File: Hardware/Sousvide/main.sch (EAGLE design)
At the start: 14 parts, among them K1 CQ1-12V, SW1 EC12E_SW, T1 2N3904

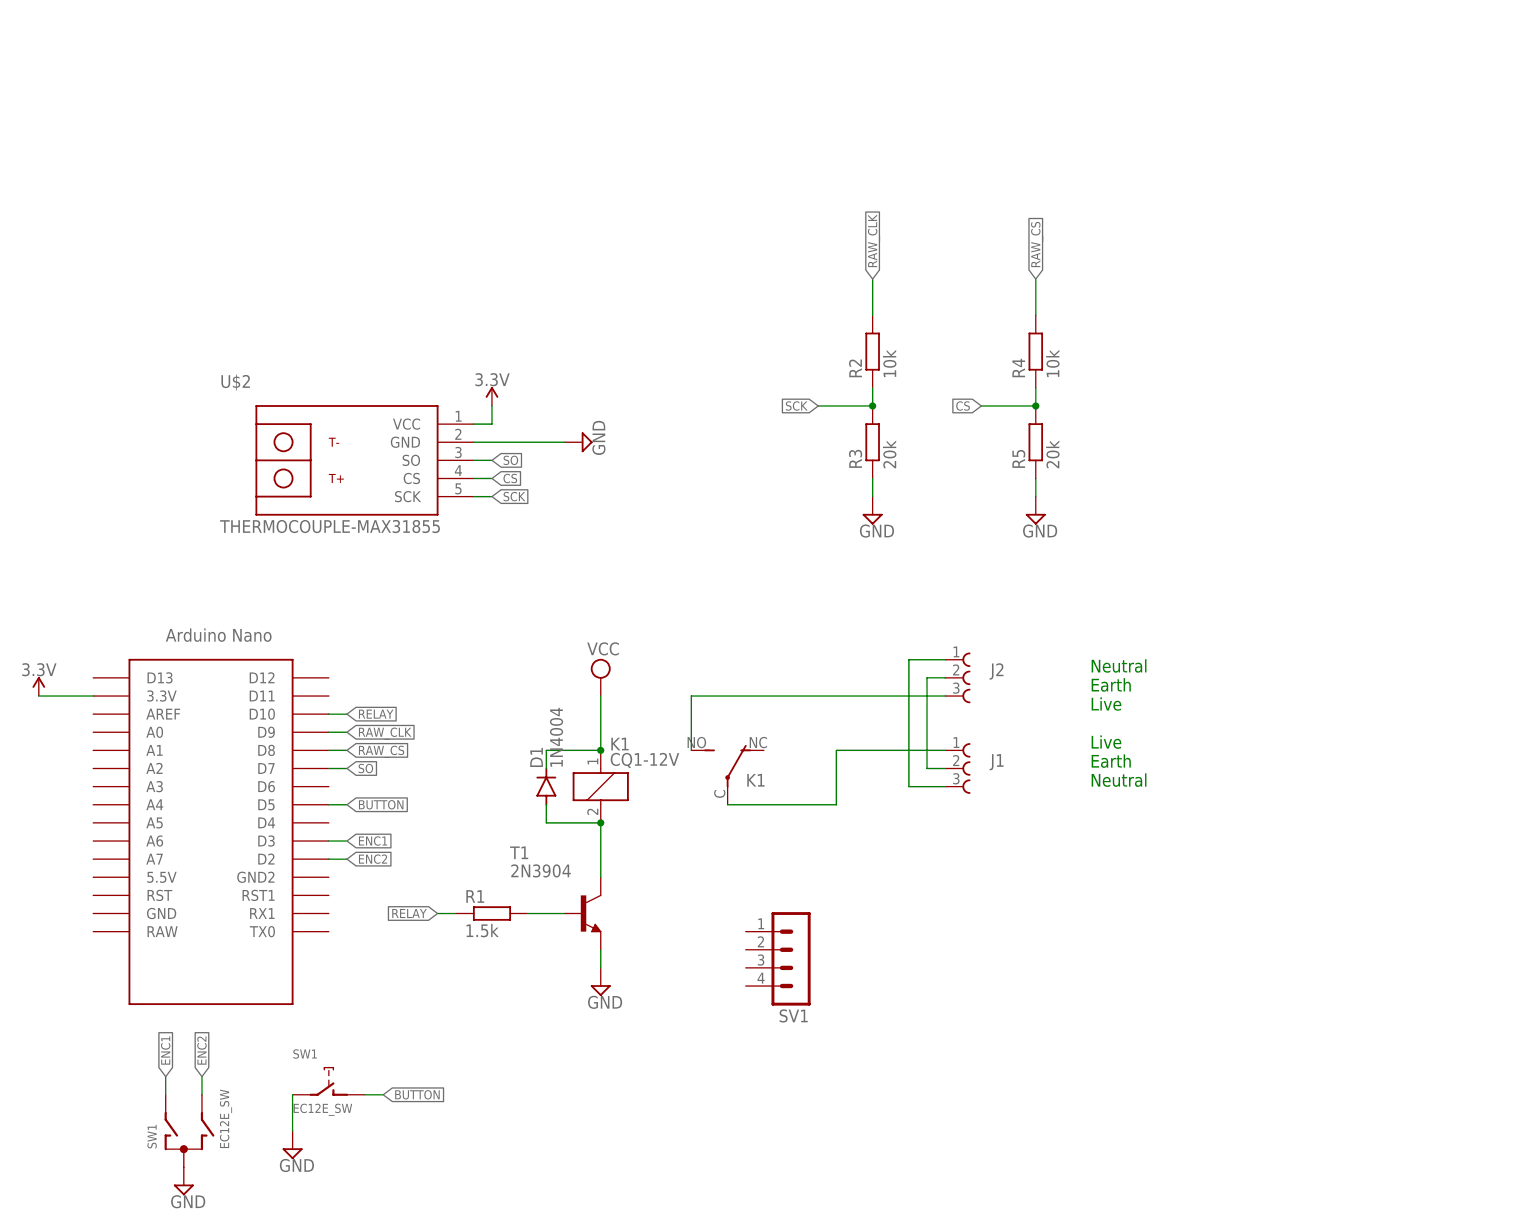
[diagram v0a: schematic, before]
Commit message: Completed schematic
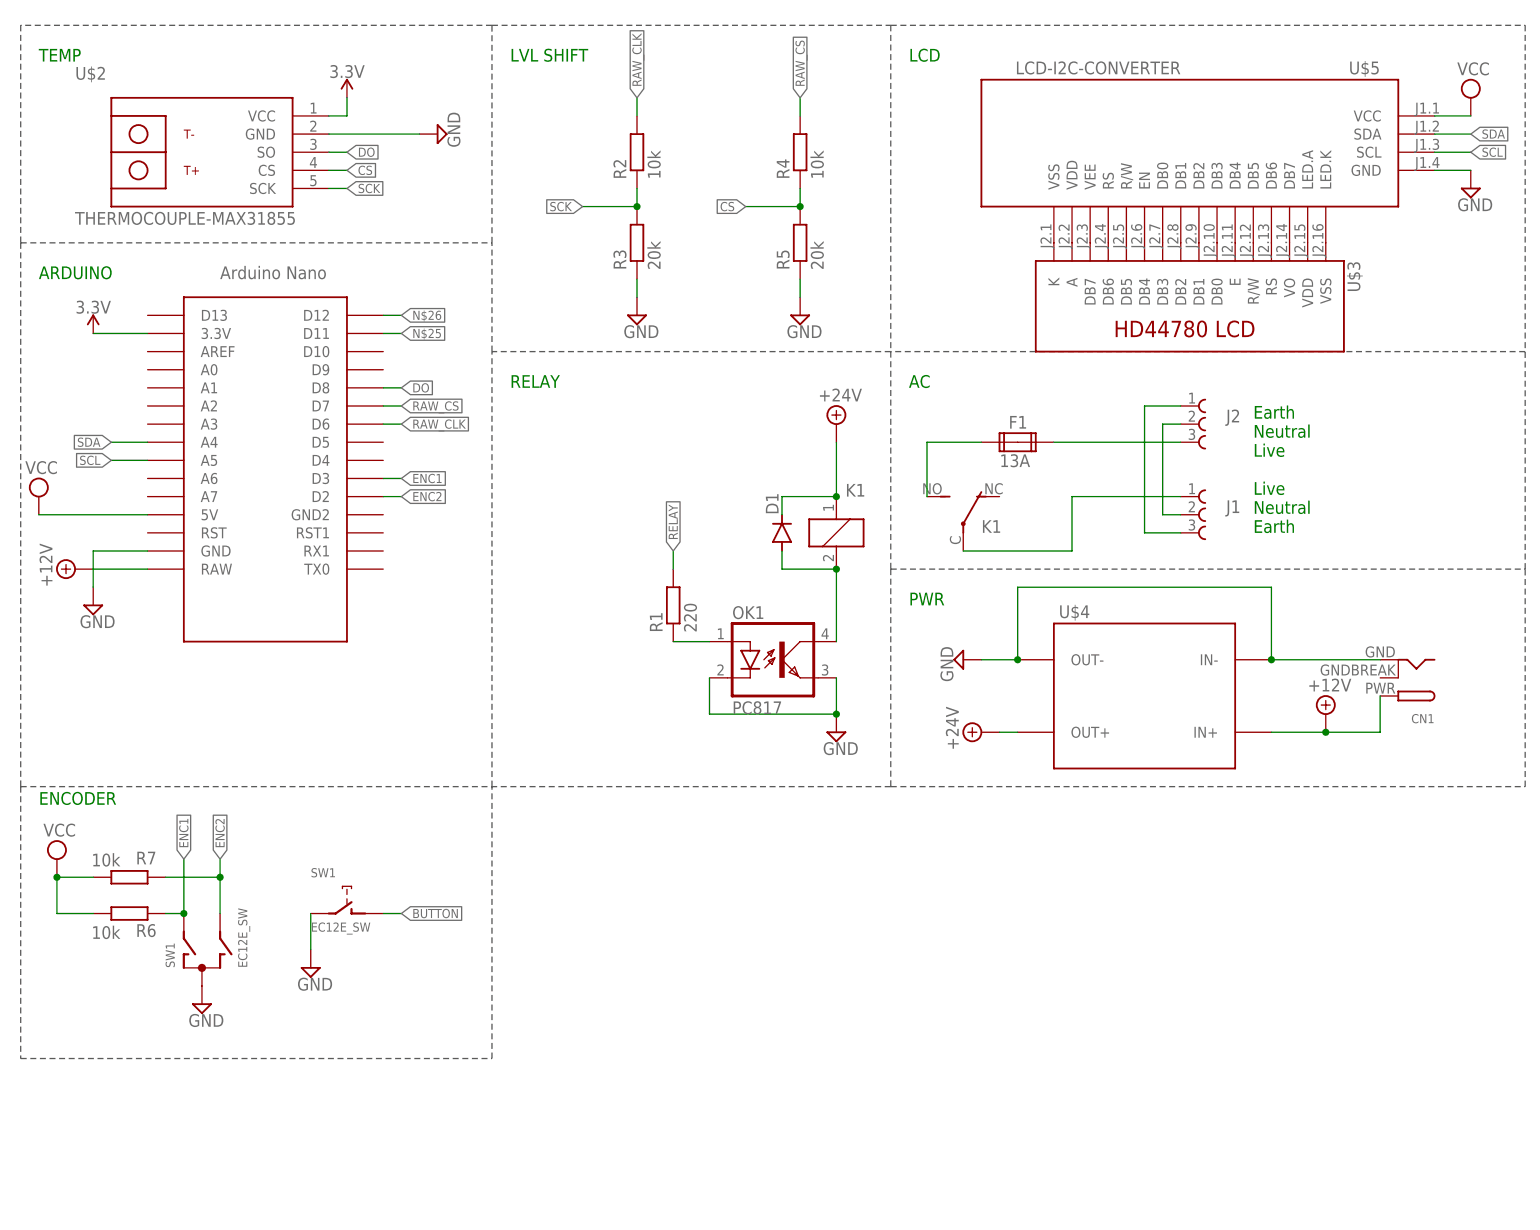
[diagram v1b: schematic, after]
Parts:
- removed SV1: (no value), con-lstb:MA04-1
- removed T1: 2N3904, transistor:2N3904
- added CN1: (no value), adafruit:DCBARRELPTH
- added F1: 13A, special:FUSE2P
- added OK1: PC817, optocoupler:PC817
- added R6, R7: 10k, rcl:R-EU_0207/7
- added U$3: LCD-HD4478016X2-4-HOLES-BL16X2-4-HOLES-BL, HD44780LCD:LCD-HD4478016X2-4-HOLES-BL16X2-4-HOLES-BL
- added U$4: DC-DC-STEP-DOWN-LM2596, i2clcd:DC-DC-STEP-DOWN-LM2596
- added U$5: LCD-I2C-CONVERTER, i2clcd:LCD-I2C-CONVERTER
- R1: value 1.5k -> 220
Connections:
- removed net SO: U$1.D7, U$2.SO
- new net +12V: CN1.PWR, U$1.RAW, U$4.IN+
- new net +24V: D1.C, K11.1, U$4.OUT+
- new net DO: U$1.D8, U$2.SO
- new net N$10: U$3.DB1, U$5.DB2
- new net N$11: U$3.DB2, U$5.DB1
- new net N$12: U$3.DB3, U$5.DB0
- new net N$13: U$3.DB4, U$5.EN
- new net N$14: U$3.DB5, U$5.R/W
- new net N$15: U$3.DB6, U$5.RS
- new net N$16: U$3.DB7, U$5.VEE
- new net N$17: U$3.E, U$5.DB4
- new net N$18: U$3.K, U$5.VSS
- new net N$19: U$3.R/W, U$5.DB5
- new net N$20: U$3.RS, U$5.DB6
- new net N$21: U$3.VDD, U$5.LED.A
- new net N$22: U$3.VO, U$5.DB7
- new net N$23: U$3.VSS, U$5.LED.K
- new net N$25: U$1.D11
- new net N$26: U$1.D12
- new net N$7: F1.2A, J2.3
- new net N$8: U$3.A, U$5.VDD
- new net N$9: U$3.DB0, U$5.DB3
- new net SCL: U$1.A5, U$5.SCL
- new net SDA: U$1.A4, U$5.SDA
- net BUTTON: no longer U$1.D5
- net ENC1: now also R6.1
- net ENC2: now also R7.1
- net GND: now also CN1.GND, OK1.C, OK1.EMIT, U$1.GND, U$4.IN-, U$4.OUT-, U$5.GND; no longer T1.E
- net N$1: now also OK1.COL; no longer T1.C
- net N$2: now also OK1.A, R1.1; no longer R1.2, T1.B
- net N$4: now also F1.1A; no longer J2.3
- net RAW_CLK: now also U$1.D6; no longer U$1.D9
- net RAW_CS: now also U$1.D7; no longer U$1.D8
- net RELAY: now also R1.2; no longer R1.1, U$1.D10
- net VCC: now also R6.2, R7.2, U$1.5V, U$5.VCC; no longer D1.C, K11.1
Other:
- note added: "AC"
- note added: "ARDUINO"
- note added: "ENCODER"
- note added: "Earth Neutral Live Live Neutral Earth"
- note added: "LCD"
- note added: "LVL SHIFT"
- note added: "PWR"
- note added: "RELAY"
- note added: "TEMP"
- note removed: "Neutral Earth Live Live Earth Neutral"
- moved on the sheet: D1, J1, J2, K1, R1, R2, R3, R4, R5, SW1, U$2
